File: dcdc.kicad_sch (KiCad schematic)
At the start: 49 parts, among them J10 Conn_01x01, J11 Conn_01x01, J12 Conn_01x01, J8 Conn_01x01, J9 Conn_01x01, T1 Transformer_SP_1S, U1 L78L33_SOT89, U2 TMP117, U3 LT3439, U6 LT3045xMSE, U7 24AA02-OT

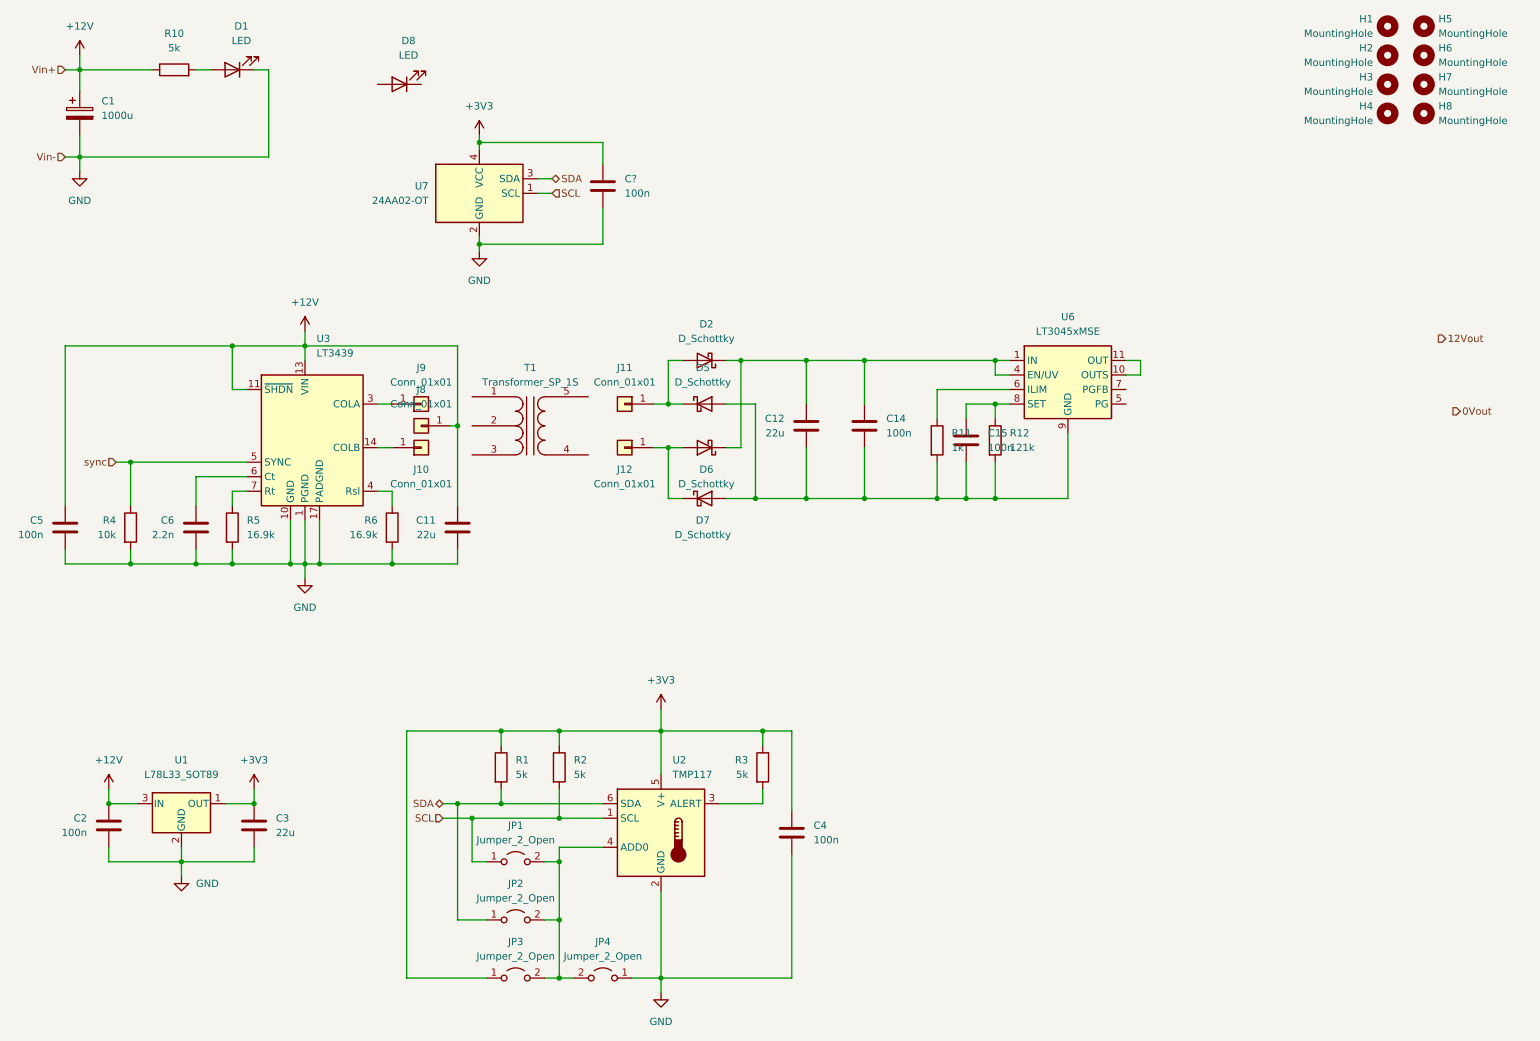
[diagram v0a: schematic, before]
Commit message: asas
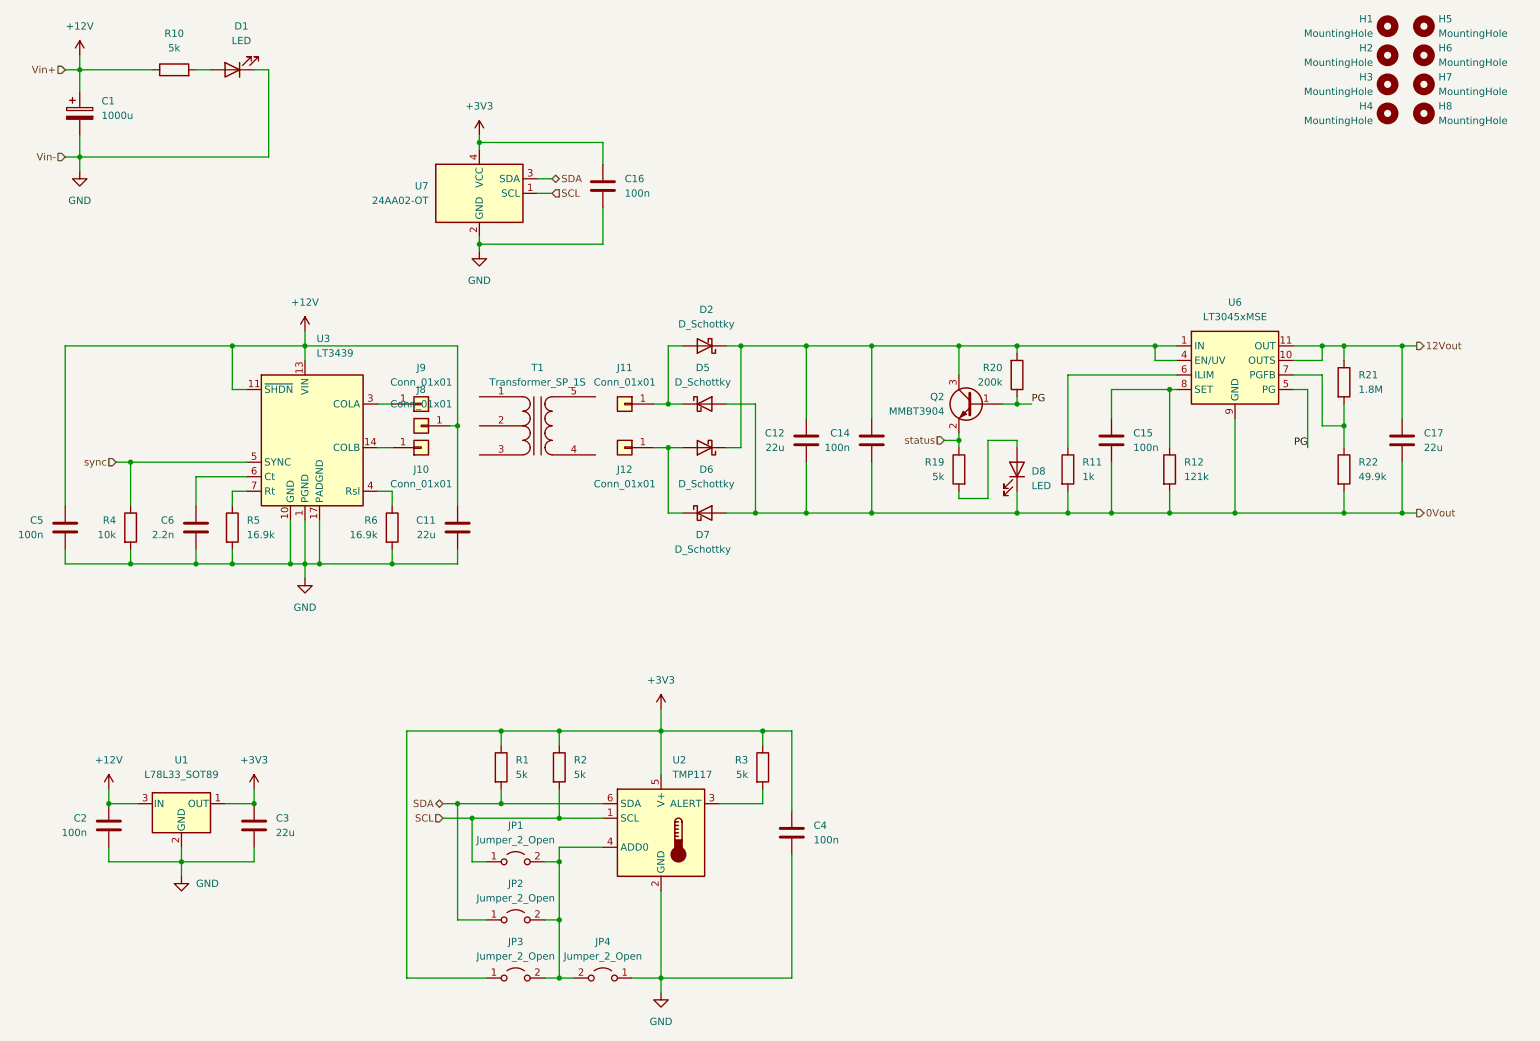
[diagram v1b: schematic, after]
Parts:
- added C17: 22u, Capacitor_SMD:C_1206_3216Metric, symbol Device:C
- added Q2: MMBT3904, Package_TO_SOT_SMD:SOT-23, symbol Transistor_BJT:MMBT3904
- added R19: 5k, Resistor_SMD:R_0805_2012Metric, symbol Device:R
- added R20: 200k, Resistor_SMD:R_0805_2012Metric, symbol Device:R
- added R21: 1.8M, Resistor_SMD:R_0805_2012Metric, symbol Device:R
- added R22: 49.9k, Resistor_SMD:R_0805_2012Metric, symbol Device:R
- gave numbers to parts that had none: 1
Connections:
- net 0Vout: now also C12.2, C14.2, C15.2, D5.2 (A), D7.2 (A), D8.1 (K), R11.2, R12.2, U6.13 (GND), U6.9 (GND), C17.2, R22.2
- net 12Vout: now also U6.10 (OUTS), U6.11 (OUT), U6.12 (OUT), C17.1, R21.1
- net at C12.1, C14.1, D2.1 (K)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: now also Q2.3 (C), R20.2
- net at D8.2 (A): now also R19.2
- net PG: now reaches U6.5 (PG)
- net PG: now also Q2.1 (B), R20.1
- net at U6.7 (PGFB): now also R21.2, R22.1
- new net status: Q2.2 (E), R19.1
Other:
- moved on the sheet: C12, C14, C15, D2, D7, D8, R11, R12, T1, U6
